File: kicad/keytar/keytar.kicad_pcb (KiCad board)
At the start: 2 copper layers, 9 parts, among them J1 DIN-5_180degree, J2 USB_B, J3 Conn_01x02, U1 Pico

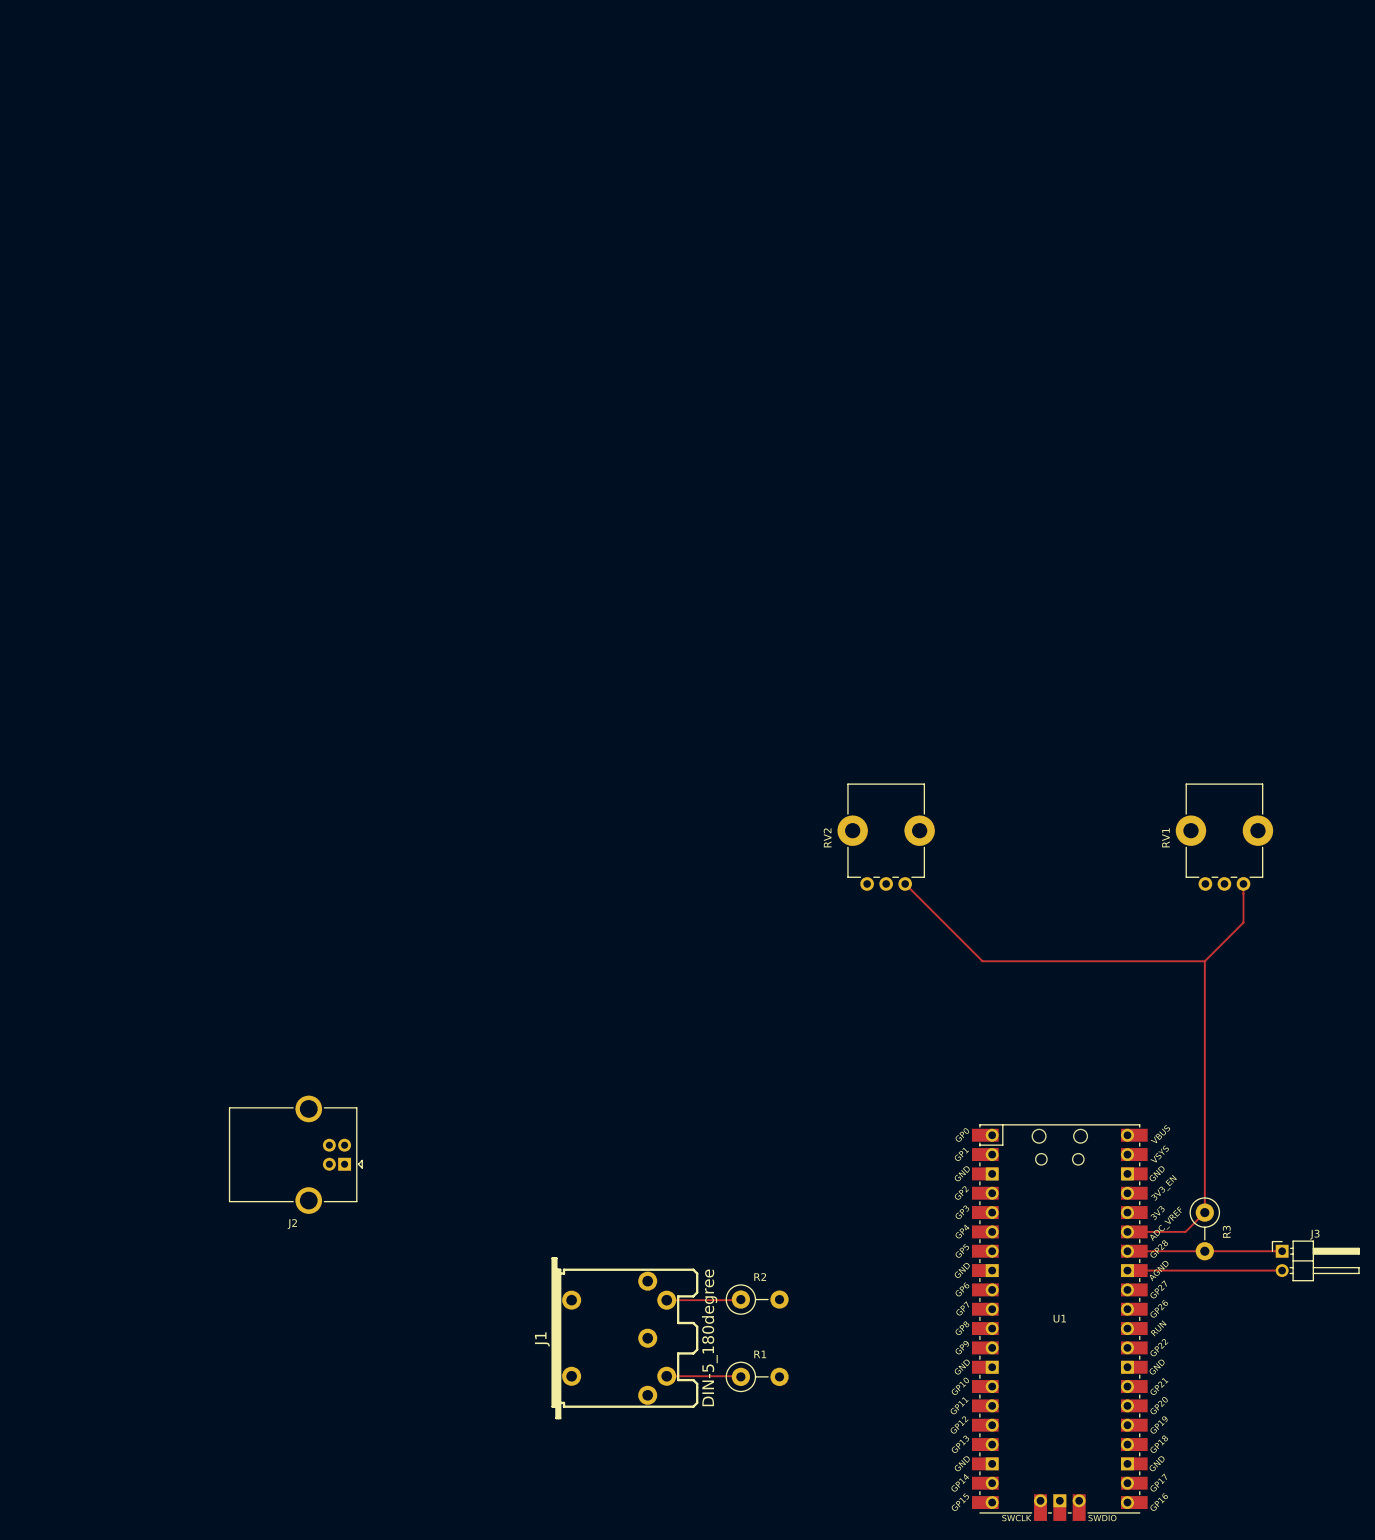
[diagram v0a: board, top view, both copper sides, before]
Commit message: properly implement PCB
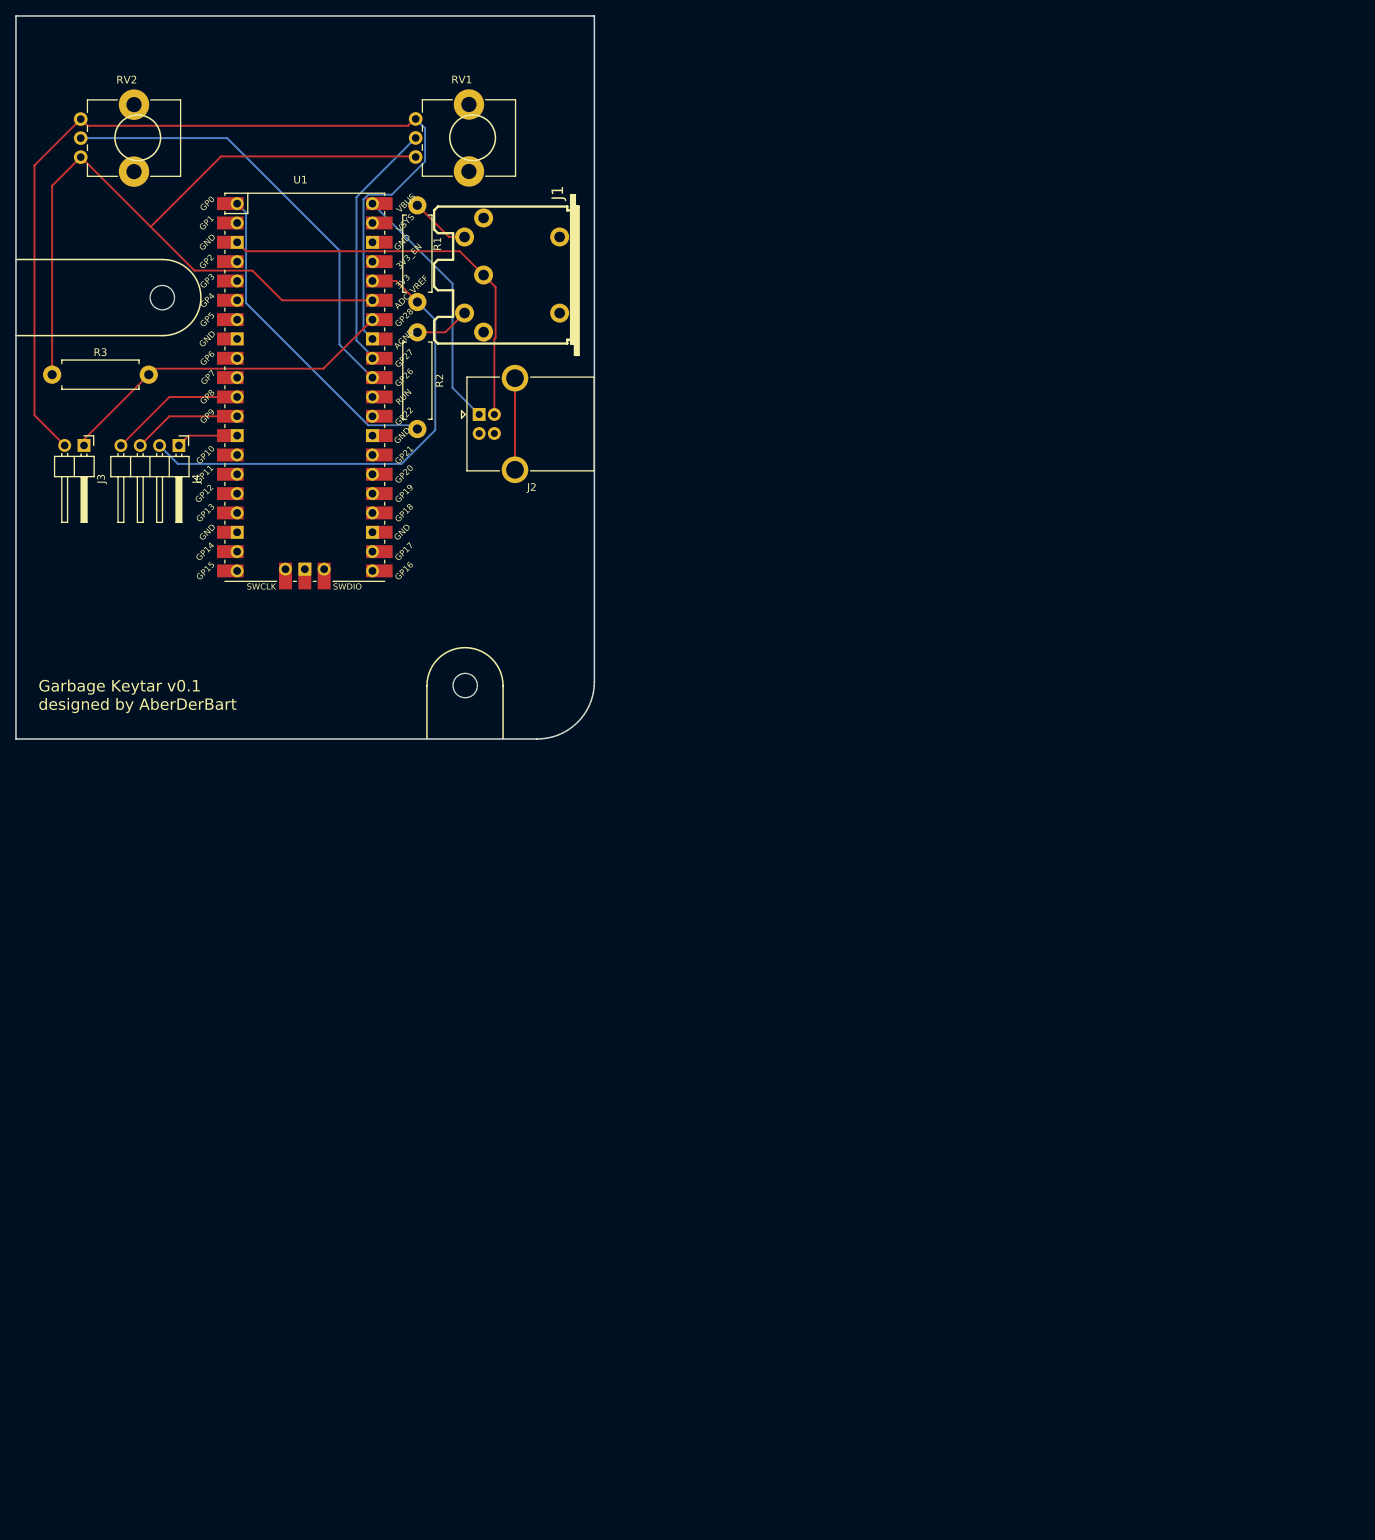
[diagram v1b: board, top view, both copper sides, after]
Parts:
- added  : MountingHole_3.2mm_M3, MountingHole:MountingHole_3.2mm_M3, F.Cu at (59.0, -7.02)
- added  : MountingHole_3.2mm_M3, MountingHole:MountingHole_3.2mm_M3, F.Cu at (19.2, -58.0)
- added J4: Conn_01x04, Connector_PinHeader_2.54mm:PinHeader_1x04_P2.54mm_Horizontal, F.Cu at (21.4, -38.6)
- J1: value DIN-5_180degree -> (none)
- R1, R2, R3: footprint Resistor_THT:R_Axial_DIN0411_L9.9mm_D3.6mm_P5.08mm_Vertical -> Resistor_THT:R_Axial_DIN0411_L9.9mm_D3.6mm_P12.70mm_Horizontal
- moved J3 189.7 mm to (8.94, -38.6), turned to 270 degrees
- moved R3 187.2 mm to (4.75, -47.9), turned to 0 degrees
- moved R1 159.7 mm to (52.7, -70.1), turned to 270 degrees
- moved U1 157.6 mm to (38.0, -46.2)
- moved RV1 144.8 mm to (52.5, -76.5), turned to 0 degrees
- moved RV2 144.4 mm to (8.51, -76.5), turned to 0 degrees
- moved J1 140.6 mm to (64.4, -61.0), turned to 90 degrees
- moved R2 134.0 mm to (52.7, -53.4), turned to 270 degrees
- moved J2 100.1 mm to (60.9, -42.6), turned to 0 degrees
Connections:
- J1 pad 2: Net-(J1-Pad2) -> GND
- U1 pad 3: Net-(J1-Pad2) -> GND
- U1 pad 38: GND -> Net-(U1-Pad38)
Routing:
- net Net-(J3-Pad2): track 20.4 -> 126.8 mm
- net Net-(J4-Pad2): track 0.00 -> 63.9 mm
- net Net-(RV2-Pad2): track 0.00 -> 58.6 mm
- net GND: track 0.00 -> 53.2 mm
- net Net-(R2-Pad2): track 0.00 -> 43.3 mm
- net Net-(J2-Pad1): track 0.00 -> 33.5 mm
- net Net-(RV1-Pad2): track 0.00 -> 33.0 mm
- net Net-(J3-Pad1): track 20.3 -> 46.3 mm
- net Net-(J4-Pad4): track 0.00 -> 17.9 mm
- net Net-(R3-Pad1): track 100.1 -> 114.9 mm
- net Net-(J4-Pad3): track 0.00 -> 14.3 mm
- net Net-(J2-Pad5): track 0.00 -> 12.0 mm
- net Net-(J4-Pad1): track 0.00 -> 8.33 mm
- net Net-(J1-Pad5): track 9.78 -> 7.25 mm
- net Net-(J1-Pad4): track 9.78 -> 7.93 mm
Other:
- board outline added: 76 x 95 mm
- board text added: "Garbage Keytar v0.1 designed by AberDerBart"
